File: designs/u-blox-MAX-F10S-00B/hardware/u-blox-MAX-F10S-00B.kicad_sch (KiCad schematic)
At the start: 0 parts

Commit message: more stuff
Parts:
- added IC101: MAX-F10S-00B, MAXF10S00B, symbol pcb-u-blox:MAX-F10S-00B
- added S101: BGS12P2L6E6327XTSA1, BGS12P2L6E6327XTSA1, symbol pcb-infineon:BGS12P2L6E6327XTSA1

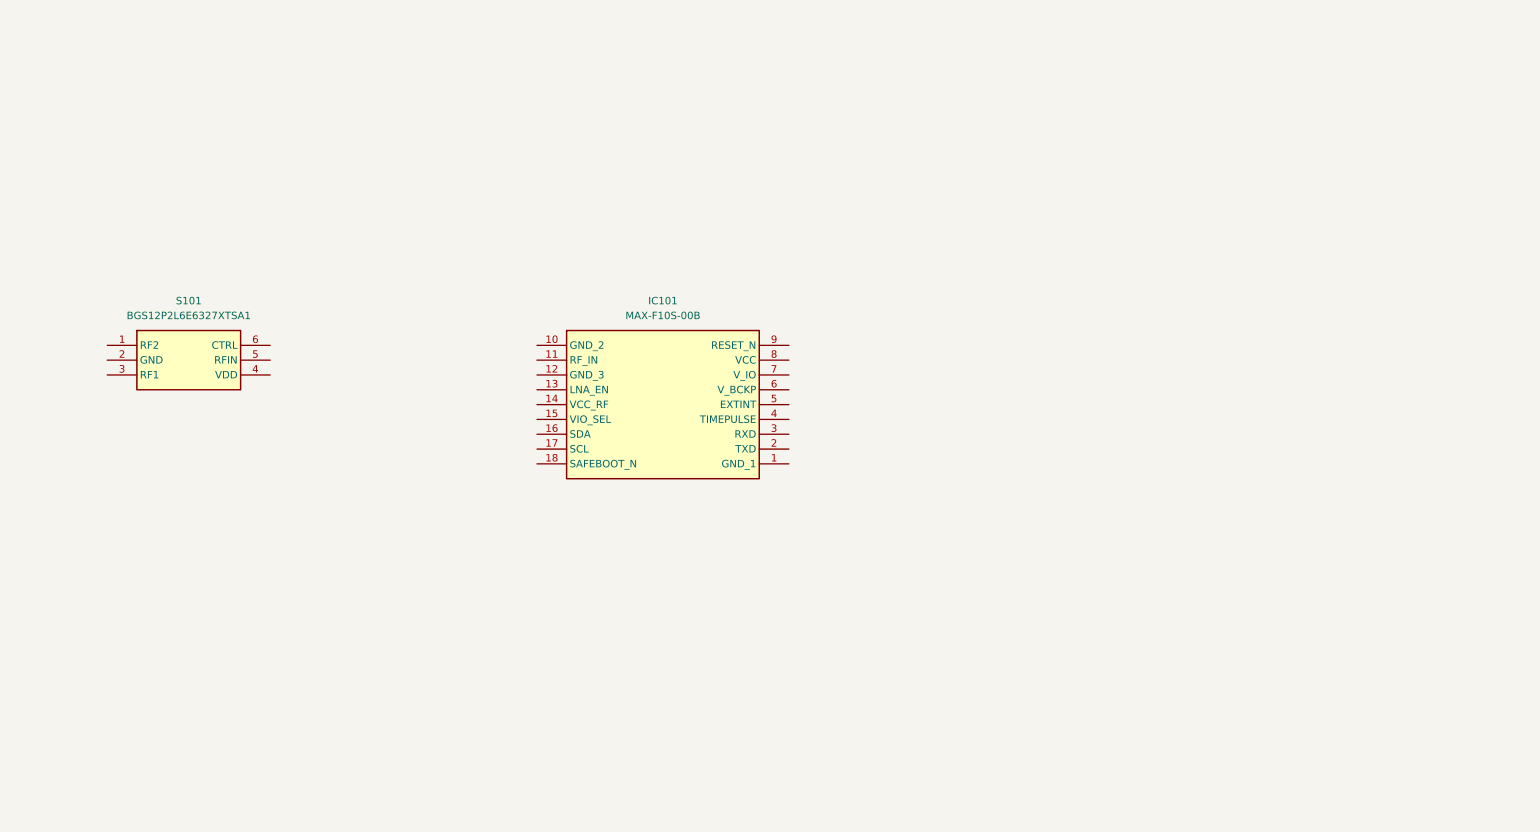
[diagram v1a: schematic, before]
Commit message: schematic done
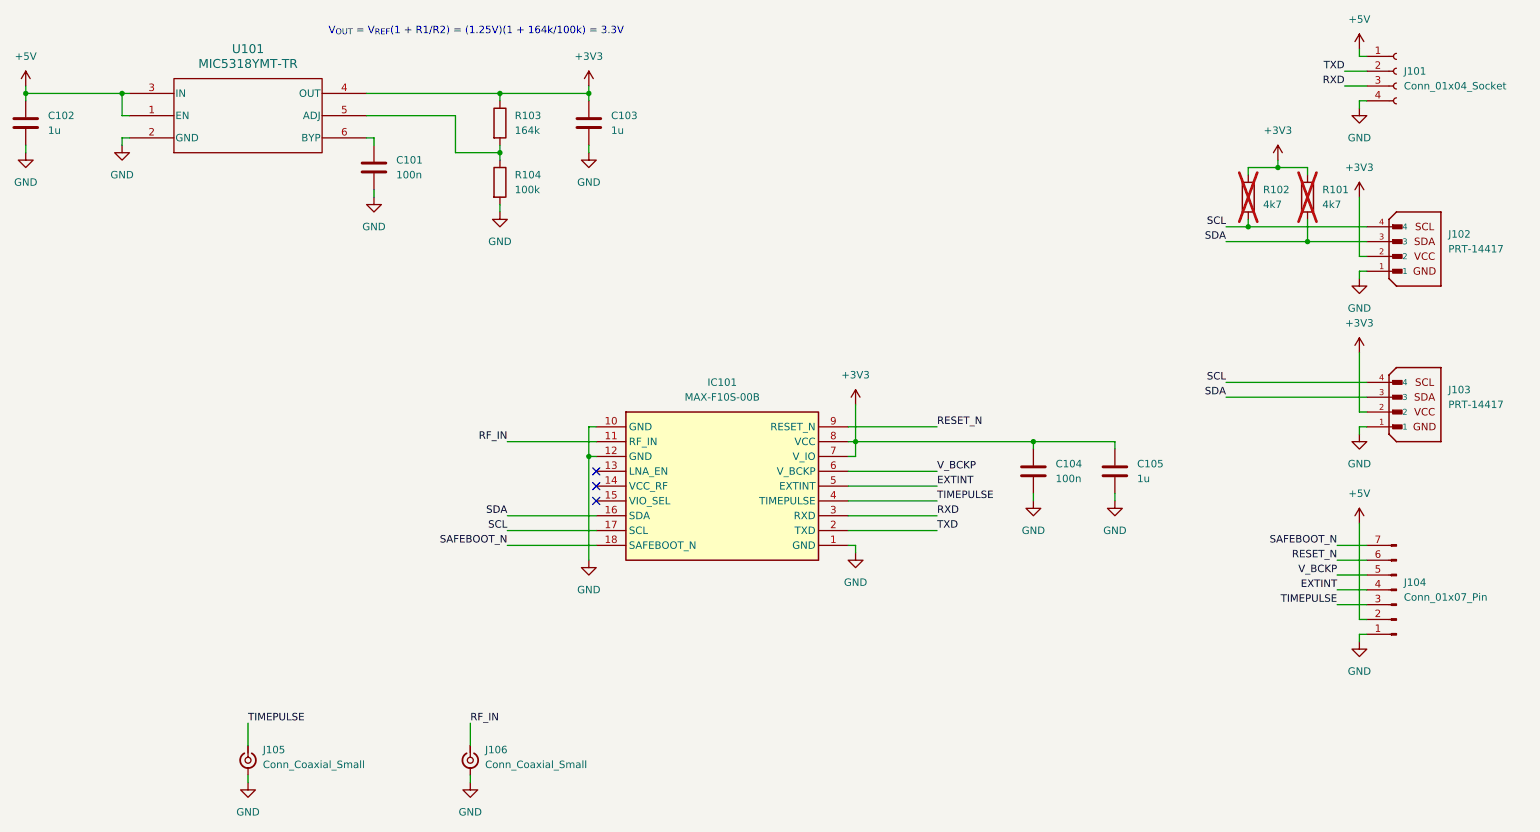
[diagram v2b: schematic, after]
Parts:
- removed S101: BGS12P2L6E6327XTSA1, BGS12P2L6E6327XTSA1, symbol pcb-infineon:BGS12P2L6E6327XTSA1
- added C101, C104: 100n, Capacitor_SMD:C_0402_1005Metric, symbol Device:C
- added C102, C103, C105: 1u, Capacitor_SMD:C_0402_1005Metric, symbol Device:C
- added J101: Conn_01x04_Socket, symbol Connector:Conn_01x04_Socket
- added J102, J103: PRT-14417, PRT-14417:SPARKFUN_PRT-14417, symbol pcb-SparkFun:PRT-14417
- added J104: Conn_01x07_Pin, symbol Connector:Conn_01x07_Pin
- added J105, J106: Conn_Coaxial_Small, Connector_Coaxial:SMA_Amphenol_132289_EdgeMount, symbol Connector:Conn_Coaxial_Small
- added R101, R102: 4k7, Resistor_SMD:R_0402_1005Metric, symbol Device:R
- added R103: 164k, Resistor_SMD:R_0402_1005Metric, symbol Device:R
- added R104: 100k, Resistor_SMD:R_0402_1005Metric, symbol Device:R
- added U101: MIC5318YMT-TR, symbol pcb-MicrochipTechnology:MIC5318YMT-TR
- IC101: footprint MAXF10S00B -> pcb-u-blox:MAXF10S00B
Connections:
- net GND: now reaches IC101.1 (GND)
- net GND: now also IC101.10 (GND), IC101.12 (GND), C101.2, C102.2, C103.2, C104.2, C105.2, J101.4 (Pin_4), J102.1, J103.1, J104.1 (Pin_1), J105.2 (Ext), J106.2 (Ext), R104.2, U101.2 (GND)
- net RF_IN: now reaches IC101.11 (RF_IN)
- net RF_IN: now also J106.1 (In)
- net SDA: now reaches IC101.16 (SDA)
- net SDA: now also J102.3, J103.3, R101.2
- net SCL: now reaches IC101.17 (SCL)
- net SCL: now also J102.4, J103.4, R102.2
- net SAFEBOOT_N: now reaches IC101.18 (SAFEBOOT_N)
- net SAFEBOOT_N: now also J104.7 (Pin_7)
- net TXD: now reaches IC101.2 (TXD)
- net TXD: now also J101.2 (Pin_2)
- net RXD: now reaches IC101.3 (RXD)
- net RXD: now also J101.3 (Pin_3)
- net TIMEPULSE: now reaches IC101.4 (TIMEPULSE)
- net TIMEPULSE: now also J104.3 (Pin_3), J105.1 (In)
- net EXTINT: now reaches IC101.5 (EXTINT)
- net EXTINT: now also J104.4 (Pin_4)
- net V_BCKP: now reaches IC101.6 (V_BCKP)
- net V_BCKP: now also J104.5 (Pin_5)
- net +3V3: now reaches IC101.7 (V_IO)
- net +3V3: now also IC101.8 (VCC), C103.1, C104.1, C105.1, J102.2, J103.2, R101.1, R102.1, R103.1, U101.4 (OUT)
- net RESET_N: now reaches IC101.9 (RESET_N)
- net RESET_N: now also J104.6 (Pin_6)
- new net: R103.2, R104.1, U101.5 (ADJ)
- new net: C101.1, U101.6 (BYP)
- new net +5V: C102.1, J101.1 (Pin_1), J104.2 (Pin_2), U101.1 (EN), U101.3 (IN)
- no-connect marks 0 -> 3
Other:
- note added: "V_{OUT} = V_{REF}(1 + R1/R2) = (1.25V)(1 + 164k/100k) = 3.3V"
